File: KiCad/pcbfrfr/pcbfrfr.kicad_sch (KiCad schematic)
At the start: 40 parts, among them J1 Barrel_Jack_Switch, J10 Conn_01x05_Pin, J11 Conn_01x05_Pin, J12 Conn_01x04_Pin, J13 Conn_01x04_Pin, J14 Conn_01x04_Pin, J15 Conn_01x04_Pin, J16 Conn_01x05_Pin, J17 Conn_01x05_Pin, J18 Conn_01x05_Pin, J19 Conn_01x05_Pin, J2 Conn_01x02_Pin, J20 Conn_01x05_Pin, J21 Conn_01x02_Pin, J3 Conn_01x19_Socket, J4 Conn_01x19_Socket, J5 Conn_01x19_Socket, J6 Conn_01x05_Pin, J7 Conn_01x19_Socket, J8 Conn_01x04_Pin, J9 Conn_01x03_Pin, U1 AP63203WU, U2 AP63205WU

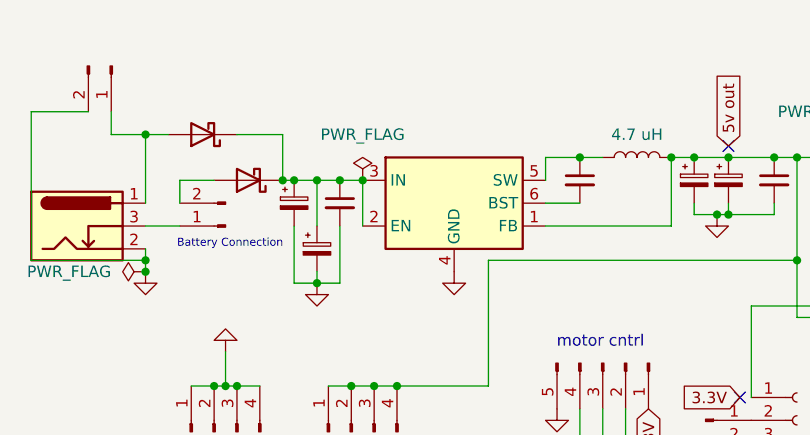
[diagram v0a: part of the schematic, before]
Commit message: newpcb
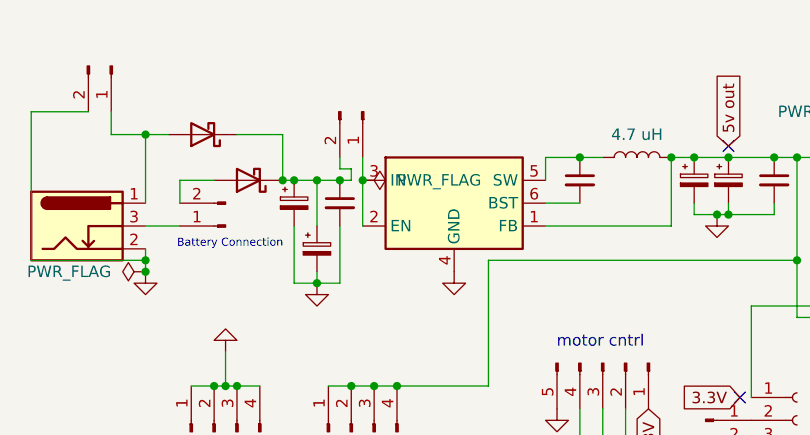
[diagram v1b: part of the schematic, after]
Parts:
- added J22: Conn_01x02_Pin, Connector_PinSocket_2.54mm:PinSocket_1x02_P2.54mm_Horizontal, symbol Connector:Conn_01x02_Pin
- J10, J11, J16, J17, J18, J19, J20, J6: footprint Connector_PinHeader_2.54mm:PinHeader_1x05_P2.54mm_Vertical -> Connector_PinSocket_2.54mm:PinSocket_1x05_P2.54mm_Vertical
- J12, J13, J14, J15, J8: footprint Connector_PinHeader_2.54mm:PinHeader_1x04_P2.54mm_Vertical -> Connector_PinSocket_2.54mm:PinSocket_1x04_P2.54mm_Vertical
- J2, J21: footprint Connector_PinHeader_2.54mm:PinHeader_1x02_P2.54mm_Vertical -> Connector_PinSocket_2.54mm:PinSocket_1x02_P2.54mm_Horizontal
- J3, J4, J5, J7: footprint Connector_PinHeader_2.54mm:PinHeader_1x19_P2.54mm_Vertical -> Connector_PinSocket_2.54mm:PinSocket_1x19_P2.54mm_Horizontal
- J9: footprint Connector_PinHeader_2.54mm:PinHeader_1x03_P2.54mm_Vertical -> Connector_PinSocket_2.54mm:PinSocket_1x03_P2.54mm_Vertical
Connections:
- net at C1.1, C5.1, C6.1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: now also J22.2 (Pin_2); no longer U2.2 (EN), U2.3 (IN)
- new net: J22.1 (Pin_1), U2.2 (EN), U2.3 (IN)
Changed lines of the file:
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@@
 	)
 	(junction
-		(at 74.93 29.21)
-		(diameter 0)
-		(color 0 0 0 0)
-	)
-	(junction
 		(at 115.57 33.02)
 		(diameter 0)
@@
 	)
 	(junction
+		(at 74.93 29.21)
+		(diameter 0)
+		(color 0 0 0 0)
+	)
+	(junction
 		(at 73.66 52.07)
 		(diameter 0)
@@
 	(wire
 		(pts
+			(xy 72.39 27.94) (xy 72.39 26.67)
+		)
+		(stroke
+			(width 0)
+			(type default)
+		)
+	)
+	(wire
+		(pts
 			(xy 223.52 77.47) (xy 153.67 77.47)
 		)
@@
 	(wire
 		(pts
+			(xy 73.66 29.21) (xy 72.39 29.21)
+		)
+		(stroke
+			(width 0)
+			(type default)
+		)
+	)
+	(wire
+		(pts
 			(xy 166.37 53.34) (xy 170.18 53.34)
 		)
@@
 	(wire
 		(pts
-			(xy 72.39 29.21) (xy 74.93 29.21)
-		)
-		(stroke
-			(width 0)
-			(type default)
-		)
-	)
-	(wire
-		(pts
 			(xy 203.2 50.8) (xy 203.2 52.07)
 		)
@@
 	(wire
 		(pts
+			(xy 73.66 29.21) (xy 73.66 27.94)
+		)
+		(stroke
+			(width 0)
+			(type default)
+		)
+	)
+	(wire
+		(pts
 			(xy 223.52 52.07) (xy 223.52 77.47)
 		)
@@
 	(wire
 		(pts
+			(xy 74.93 26.67) (xy 74.93 29.21)
+		)
+		(stroke
+			(width 0)
+			(type default)
+		)
+	)
+	(wire
+		(pts
 			(xy 179.07 46.99) (xy 184.15 46.99)
 		)
@@
 	(wire
 		(pts
+			(xy 73.66 27.94) (xy 72.39 27.94)
+		)
+		(stroke
+			(width 0)
+			(type default)
+		)
+	)
+	(wire
+		(pts
 			(xy 153.67 59.69) (xy 153.67 58.42)
 		)
@@
 	(wire
 		(pts
+			(xy 74.93 29.21) (xy 74.93 34.29)
+		)
+		(stroke
+			(width 0)
+			(type default)
+		)
+	)
+	(wire
+		(pts
 			(xy 194.31 82.55) (xy 151.13 82.55)
 		)
@@
 	(wire
 		(pts
-			(xy 74.93 29.21) (xy 74.93 34.29)
-		)
-		(stroke
-			(width 0)
-			(type default)
-		)
-	)
-	(wire
-		(pts
 			(xy 190.5 59.69) (xy 153.67 59.69)
 		)
@@
 			)
 		)
-		(property "Footprint" "Connector_PinHeader_2.54mm:PinHeader_1x05_P2.54mm_Vertical"
+		(property "Footprint" "Connector_PinSocket_2.54mm:PinSocket_1x05_P2.54mm_Vertical"
 			(at 139.7 62.23 0)
 			(effects
@@
 	)
 	(symbol
+		(lib_id "Connector:Conn_01x02_Pin")
+		(at 74.93 21.59 270)
+		(unit 1)
+		(exclude_from_sim no)
+		(in_bom yes)
+		(on_board yes)
+		(dnp no)
+		(fields_autoplaced yes)
+		(property "Reference" "J22"
+			(at 76.2 20.9549 90)
+			(effects
+				(font
+					(size 1.27 1.27)
+				)
+				(justify left)
+				(hide yes)
+			)
+		)
+		(property "Value" "Conn_01x02_Pin"
+			(at 76.2 23.4949 90)
+			(effects
+				(font
+					(size 1.27 1.27)
+				)
+				(justify left)
+				(hide yes)
+			)
+		)
+		(property "Footprint" "Connector_PinSocket_2.54mm:PinSocket_1x02_P2.54mm_Horizontal"
+			(at 74.93 21.59 0)
+			(effects
+				(font
+					(size 1.27 1.27)
+				)
+				(hide yes)
+			)
+		)
+		(property "Datasheet" "~"
+			(at 74.93 21.59 0)
+			(effects
+				(font
+					(size 1.27 1.27)
+				)
+				(hide yes)
+			)
+		)
+		(property "Description" "Generic connector, single row, 01x02, script generated"
+			(at 74.93 21.59 0)
+			(effects
+				(font
+					(size 1.27 1.27)
+				)
+				(hide yes)
+			)
+		)
+		(pin "1"
+		)
+		(pin "2"
+		)
+		(instances
+			(project "pcbfrfr"
+				(path "/c57ab67e-e0d3-4941-87dd-e1b23ac81707"
+					(reference "J22")
+					(unit 1)
+				)
+			)
+		)
+	)
+	(symbol
 		(lib_id "Connector:Conn_01x04_Pin")
 		(at 187.96 13.97 270)
@@
 			)
 		)
-		(property "Footprint" "Connector_PinHeader_2.54mm:PinHeader_1x04_P2.54mm_Vertical"
+		(property "Footprint" "Connector_PinSocket_2.54mm:PinSocket_1x04_P2.54mm_Vertical"
 			(at 187.96 13.97 0)
 			(effects
@@
 			)
 		)
-		(property "Footprint" "Connector_PinHeader_2.54mm:PinHeader_1x05_P2.54mm_Vertical"
+		(property "Footprint" "Connector_PinSocket_2.54mm:PinSocket_1x05_P2.54mm_Vertical"
 			(at 113.03 73.66 0)
 			(effects
@@
 			)
 		)
-		(property "Footprint" "Connector_PinHeader_2.54mm:PinHeader_1x05_P2.54mm_Vertical"
+		(property "Footprint" "Connector_PinSocket_2.54mm:PinSocket_1x05_P2.54mm_Vertical"
 			(at 180.34 67.31 0)
 			(effects
@@
 			)
 		)
-		(property "Footprint" "Connector_PinHeader_2.54mm:PinHeader_1x02_P2.54mm_Vertical"
+		(property "Footprint" "Connector_PinSocket_2.54mm:PinSocket_1x02_P2.54mm_Horizontal"
 			(at 46.99 16.51 0)
 			(effects
@@
 			)
 		)
-		(property "Footprint" "Connector_PinHeader_2.54mm:PinHeader_1x05_P2.54mm_Vertical"
+		(property "Footprint" "Connector_PinSocket_2.54mm:PinSocket_1x05_P2.54mm_Vertical"
 			(at 135.89 60.96 0)
 			(effects
@@
 			)
 		)
-		(property "Footprint" "Connector_PinHeader_2.54mm:PinHeader_1x05_P2.54mm_Vertical"
+		(property "Footprint" "Connector_PinSocket_2.54mm:PinSocket_1x05_P2.54mm_Vertical"
 			(at 113.03 60.96 0)
 			(effects
@@
 			)
 		)
-		(property "Footprint" "Connector_PinHeader_2.54mm:PinHeader_1x02_P2.54mm_Vertical"
+		(property "Footprint" "Connector_PinSocket_2.54mm:PinSocket_1x02_P2.54mm_Horizontal"
 			(at 59.69 34.29 0)
 			(effects
@@
 			)
 		)
-		(property "Footprint" "Connector_PinHeader_2.54mm:PinHeader_1x19_P2.54mm_Vertical"
+		(property "Footprint" "Connector_PinSocket_2.54mm:PinSocket_1x19_P2.54mm_Horizontal"
 			(at 123.19 76.2 0)
 			(effects
@@
 	(symbol
 		(lib_id "power:PWR_FLAG")
-		(at 74.93 29.21 0)
+		(at 74.93 29.21 270)
 		(unit 1)
 		(exclude_from_sim no)
@@
 		(fields_autoplaced yes)
 		(property "Reference" "#FLG01"
-			(at 74.93 27.305 0)
+			(at 76.835 29.21 0)
 			(effects
 				(font
@@
 		)
 		(property "Value" "PWR_FLAG"
-			(at 74.93 24.13 0)
+			(at 78.74 29.2099 90)
 			(effects
 				(font
 					(size 1.27 1.27)
 				)
+				(justify left)
 			)
 		)
@@
 			)
 		)
-		(property "Footprint" "Connector_PinHeader_2.54mm:PinHeader_1x05_P2.54mm_Vertical"
+		(property "Footprint" "Connector_PinSocket_2.54mm:PinSocket_1x05_P2.54mm_Vertical"
 			(at 194.31 74.93 0)
 			(effects
@@
 			)
 		)
-		(property "Footprint" "Connector_PinHeader_2.54mm:PinHeader_1x04_P2.54mm_Vertical"
+		(property "Footprint" "Connector_PinSocket_2.54mm:PinSocket_1x04_P2.54mm_Vertical"
 			(at 73.66 57.15 0)
 			(effects
@@
 			)
 		)
-		(property "Footprint" "Connector_PinHeader_2.54mm:PinHeader_1x19_P2.54mm_Vertical"
+		(property "Footprint" "Connector_PinSocket_2.54mm:PinSocket_1x19_P2.54mm_Horizontal"
 			(at 161.29 76.2 0)
 			(effects
@@
 			)
 		)
-		(property "Footprint" "Connector_PinHeader_2.54mm:PinHeader_1x04_P2.54mm_Vertical"
+		(property "Footprint" "Connector_PinSocket_2.54mm:PinSocket_1x04_P2.54mm_Vertical"
 			(at 176.53 17.78 0)
 			(effects
@@
 			)
 		)
-		(property "Footprint" "Connector_PinHeader_2.54mm:PinHeader_1x04_P2.54mm_Vertical"
+		(property "Footprint" "Connector_PinSocket_2.54mm:PinSocket_1x04_P2.54mm_Vertical"
 			(at 58.42 57.15 0)
 			(effects
@@
 			)
 		)
-		(property "Footprint" "Connector_PinHeader_2.54mm:PinHeader_1x05_P2.54mm_Vertical"
+		(property "Footprint" "Connector_PinSocket_2.54mm:PinSocket_1x05_P2.54mm_Vertical"
 			(at 222.25 43.18 0)
 			(effects
@@
 			)
 		)
-		(property "Footprint" "Connector_PinHeader_2.54mm:PinHeader_1x04_P2.54mm_Vertical"
+		(property "Footprint" "Connector_PinSocket_2.54mm:PinSocket_1x04_P2.54mm_Vertical"
 			(at 186.69 44.45 0)
 			(effects
@@
 			)
 		)
-		(property "Footprint" "Connector_PinHeader_2.54mm:PinHeader_1x19_P2.54mm_Vertical"
+		(property "Footprint" "Connector_PinSocket_2.54mm:PinSocket_1x19_P2.54mm_Horizontal"
 			(at 125.73 76.2 0)
 			(effects
@@
 			)
 		)
-		(property "Footprint" "Connector_PinHeader_2.54mm:PinHeader_1x03_P2.54mm_Vertical"
+		(property "Footprint" "Connector_PinSocket_2.54mm:PinSocket_1x03_P2.54mm_Vertical"
 			(at 204.47 43.18 0)
 			(effects
@@
 			)
 		)
-		(property "Footprint" "Connector_PinHeader_2.54mm:PinHeader_1x19_P2.54mm_Vertical"
+		(property "Footprint" "Connector_PinSocket_2.54mm:PinSocket_1x19_P2.54mm_Horizontal"
 			(at 158.75 76.2 0)
 			(effects
@@
 			)
 		)
-		(property "Footprint" "Connector_PinHeader_2.54mm:PinHeader_1x05_P2.54mm_Vertical"
+		(property "Footprint" "Connector_PinSocket_2.54mm:PinSocket_1x05_P2.54mm_Vertical"
 			(at 101.6 49.53 0)
 			(effects

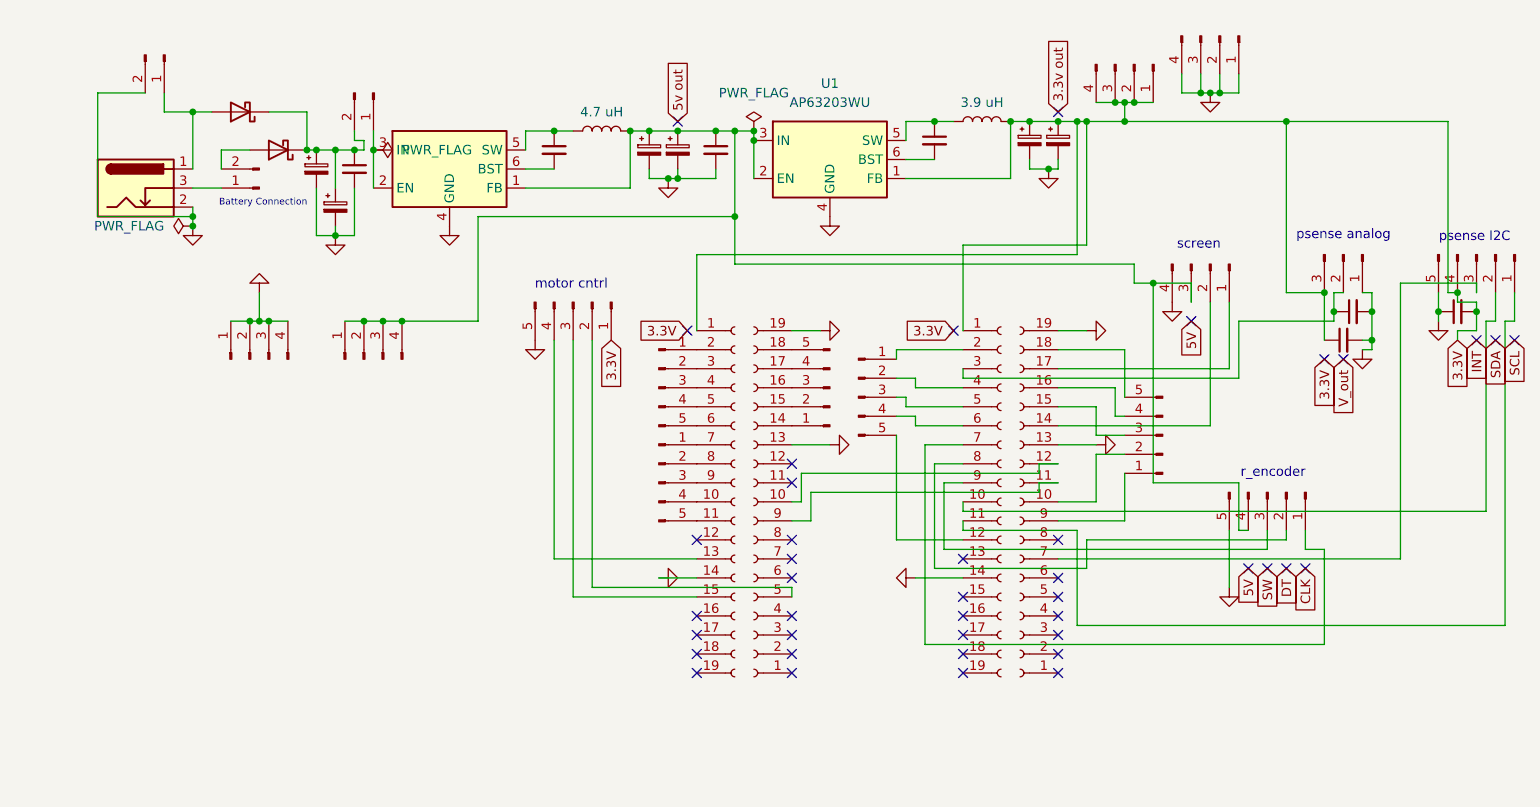
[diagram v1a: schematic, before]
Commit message: updatedpcb
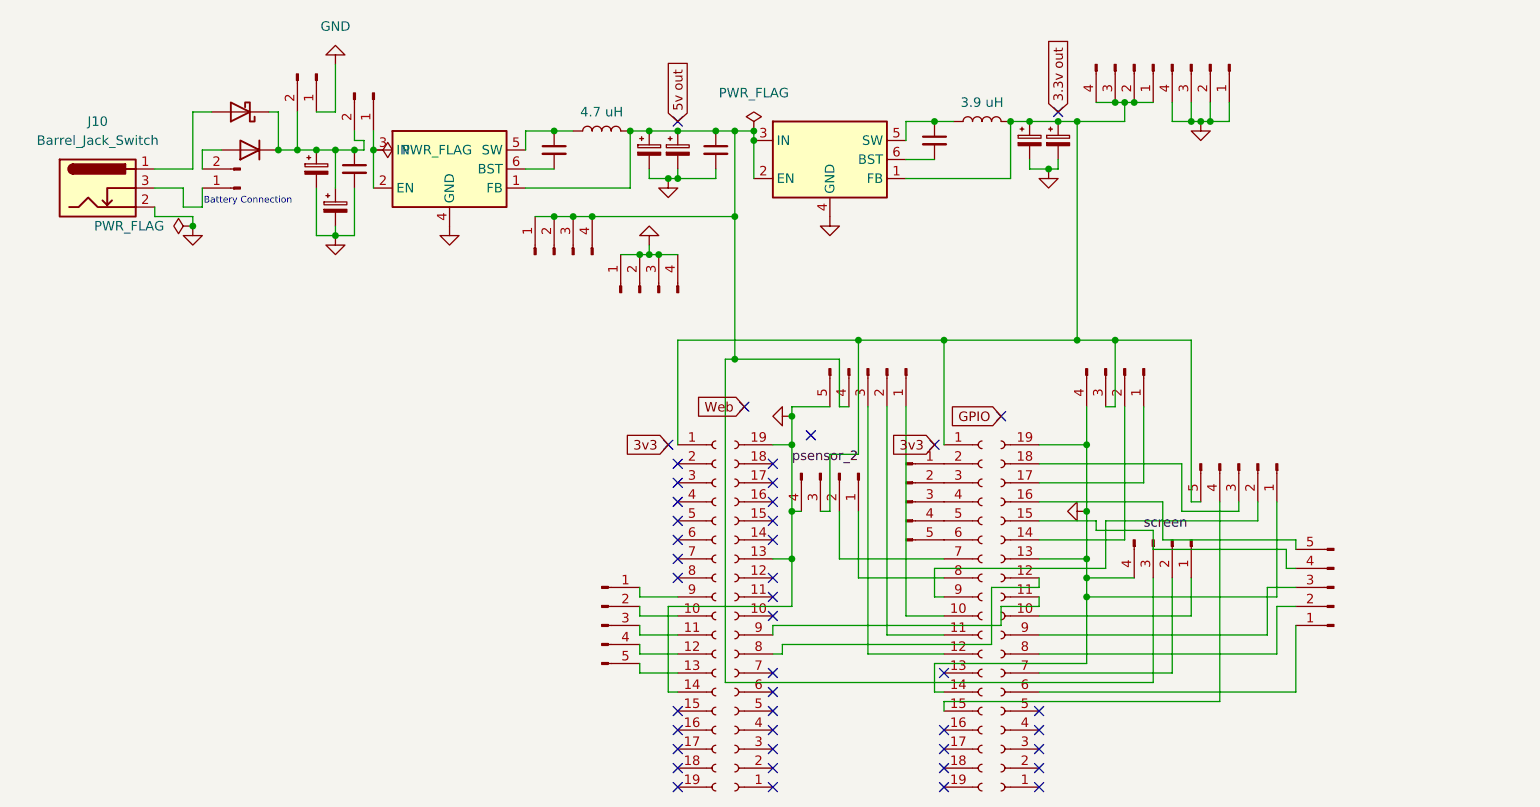
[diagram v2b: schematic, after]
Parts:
- removed C11: 0.001 uF, Capacitor_SMD:C_0402_1005Metric, symbol Device:C_Small
- removed C12, C13: 0.1 uF, Capacitor_SMD:C_0402_1005Metric, symbol Device:C_Small
- removed D1: SS24, Diode_SMD:D_SMA, symbol Diode:SS24
- removed J1: Barrel_Jack_Switch, Connector_BarrelJack:BarrelJack_CLIFF_FC681465S_SMT_Horizontal, symbol Connector:Barrel_Jack_Switch
- removed J10, J19, J20, J6: Conn_01x05_Pin, Connector_PinSocket_2.54mm:PinSocket_1x05_P2.54mm_Vertical, symbol Connector:Conn_01x05_Pin
- removed J9: Conn_01x03_Pin, Connector_PinSocket_2.54mm:PinSocket_1x03_P2.54mm_Vertical, symbol Connector:Conn_01x03_Pin
- added D2: US2AA, Diode_SMD:D_SMA, symbol Diode:US2AA
- added J1: Conn_01x05_Pin, Connector_PinHeader_2.54mm:PinHeader_1x05_P2.54mm_Vertical, symbol Connector:Conn_01x05_Pin
- added J10: Barrel_Jack_Switch, Connector_BarrelJack:BarrelJack_CLIFF_FC681465S_SMT_Horizontal, symbol Connector:Barrel_Jack_Switch
- added J6, J9: Conn_01x04_Pin, Connector_PinHeader_2.54mm:PinHeader_1x04_P2.54mm_Vertical, symbol Connector:Conn_01x04_Pin
- J11, J16, J17, J18: footprint Connector_PinSocket_2.54mm:PinSocket_1x05_P2.54mm_Vertical -> Connector_PinHeader_2.54mm:PinHeader_1x05_P2.54mm_Vertical
- J12, J13, J14, J15, J8: footprint Connector_PinSocket_2.54mm:PinSocket_1x04_P2.54mm_Vertical -> Connector_PinHeader_2.54mm:PinHeader_1x04_P2.54mm_Vertical
- J2: value Conn_01x02_Pin -> battery; footprint Connector_PinSocket_2.54mm:PinSocket_1x02_P2.54mm_Horizontal -> Connector_PinHeader_2.54mm:PinHeader_1x02_P2.54mm_Vertical
- J21: value Conn_01x02_Pin -> mtr; footprint Connector_PinSocket_2.54mm:PinSocket_1x02_P2.54mm_Horizontal -> Connector_PinHeader_2.54mm:PinHeader_1x02_P2.54mm_Vertical
- J22: value Conn_01x02_Pin -> estop; footprint Connector_PinSocket_2.54mm:PinSocket_1x02_P2.54mm_Horizontal -> Connector_PinHeader_2.54mm:PinHeader_1x02_P2.54mm_Vertical
- J3, J4, J5, J7: footprint Connector_PinSocket_2.54mm:PinSocket_1x19_P2.54mm_Horizontal -> Connector_PinHeader_2.54mm:PinHeader_1x19_P2.54mm_Vertical
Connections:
- net GND: now also J11.1 (Pin_1), J21.1 (Pin_1), J1.5 (Pin_5), J10.2, J6.4 (Pin_4), J9.4 (Pin_4); no longer J11.5 (Pin_5), J21.2 (Pin_2)
- net at J4.2 (Pin_2): now also J16.1 (Pin_1)
- net at J4.4 (Pin_4): now also J16.3 (Pin_3)
- net at J4.5 (Pin_5): now also J16.4 (Pin_4)
- net at J4.6 (Pin_6): now also J16.5 (Pin_5)
- net at J4.12 (Pin_12): now also J1.3 (Pin_3)
- net at C1.1, C5.1, C6.1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: now also J21.2 (Pin_2), D2.1 (K)
- net at J17.1 (Pin_1): now also J5.6 (Pin_6); no longer J3.7 (Pin_7)
- net at J17.2 (Pin_2): now also J5.8 (Pin_8); no longer J3.8 (Pin_8)
- net at J17.3 (Pin_3): now also J5.9 (Pin_9); no longer J3.9 (Pin_9)
- net at J3.10 (Pin_10): now also J18.2 (Pin_2); no longer J17.4 (Pin_4)
- net at J17.5 (Pin_5): now also J5.16 (Pin_16); no longer J3.11 (Pin_11)
- net at D3.2 (A): now also J10.1; no longer J21.1 (Pin_1)
- net at J2.1 (Pin_1): now also J10.3
- net at C3.1, C4.1, C7.1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: now also J1.4 (Pin_4), J9.3 (Pin_3); no longer J11.4 (Pin_4), J8.3 (Pin_3)
- net at J5.10 (Pin_10): now also J9.1 (Pin_1)
- net screen: now reaches J5.15 (Pin_15)
- net screen: now also J17.4 (Pin_4)
- net at J5.18 (Pin_18): now also J11.3 (Pin_3)
- net at J18.1 (Pin_1): now also J3.9 (Pin_9); no longer J7.14 (Pin_14)
- net at J7.15 (Pin_15): no longer J18.2 (Pin_2)
- net at J18.3 (Pin_3): now also J3.11 (Pin_11); no longer J7.16 (Pin_16)
- net at J18.4 (Pin_4): now also J3.12 (Pin_12); no longer J7.17 (Pin_17)
- net at J18.5 (Pin_5): now also J3.13 (Pin_13); no longer J7.18 (Pin_18)
- net at J2.2 (Pin_2): now also D2.2 (A)
- net at J3.2 (Pin_2): no longer J16.1 (Pin_1)
- net at J3.3 (Pin_3): no longer J16.2 (Pin_2)
- net at J3.4 (Pin_4): no longer J16.3 (Pin_3)
- net at J3.5 (Pin_5): no longer J16.4 (Pin_4)
- net at J3.6 (Pin_6): no longer J16.5 (Pin_5)
- net at J4.7 (Pin_7): now also J8.2 (Pin_2); no longer J11.1 (Pin_1)
- net at J11.2 (Pin_2): now also J4.9 (Pin_9); no longer J4.8 (Pin_8)
- net at J5.12 (Pin_12): now also J7.8 (Pin_8); no longer J7.10 (Pin_10)
- net at J5.14 (Pin_14): now also J6.2 (Pin_2); no longer J8.2 (Pin_2)
- net at J5.17 (Pin_17): now also J6.1 (Pin_1); no longer J8.1 (Pin_1)
- net at J5.7 (Pin_7): now also J9.2 (Pin_2)
- net at J4.11 (Pin_11): now also J1.2 (Pin_2)
- net at J4.10 (Pin_10): now also J1.1 (Pin_1)
- net at J4.3 (Pin_3): now also J16.2 (Pin_2)
- net at J4.15 (Pin_15): now also J11.4 (Pin_4)
- net 3.3V: no longer names the net of C10.1, C9.1, J14.1 (Pin_1), J14.2 (Pin_2), J14.3 (Pin_3), J14.4 (Pin_4), J3.1 (Pin_1), J4.1 (Pin_1), L3.2, U1.1 (FB)
- net 3.3V: now also J11.5 (Pin_5), J8.3 (Pin_3), J6.3 (Pin_3)
- new net: J4.8 (Pin_8), J8.1 (Pin_1)
- no-connect marks 41 -> 44
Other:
- note removed: "motor cntrl"
- note removed: "psense I2C"
- note removed: "psense analog"
- note removed: "r_encoder"
- note removed: "screen"
